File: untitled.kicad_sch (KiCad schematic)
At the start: 6 parts, among them J13 HDMI_A_1.4, J3 Bus_M.2_Socket_M, J5 USB3_A, J6 USB3_A, M1 M.2 Screw

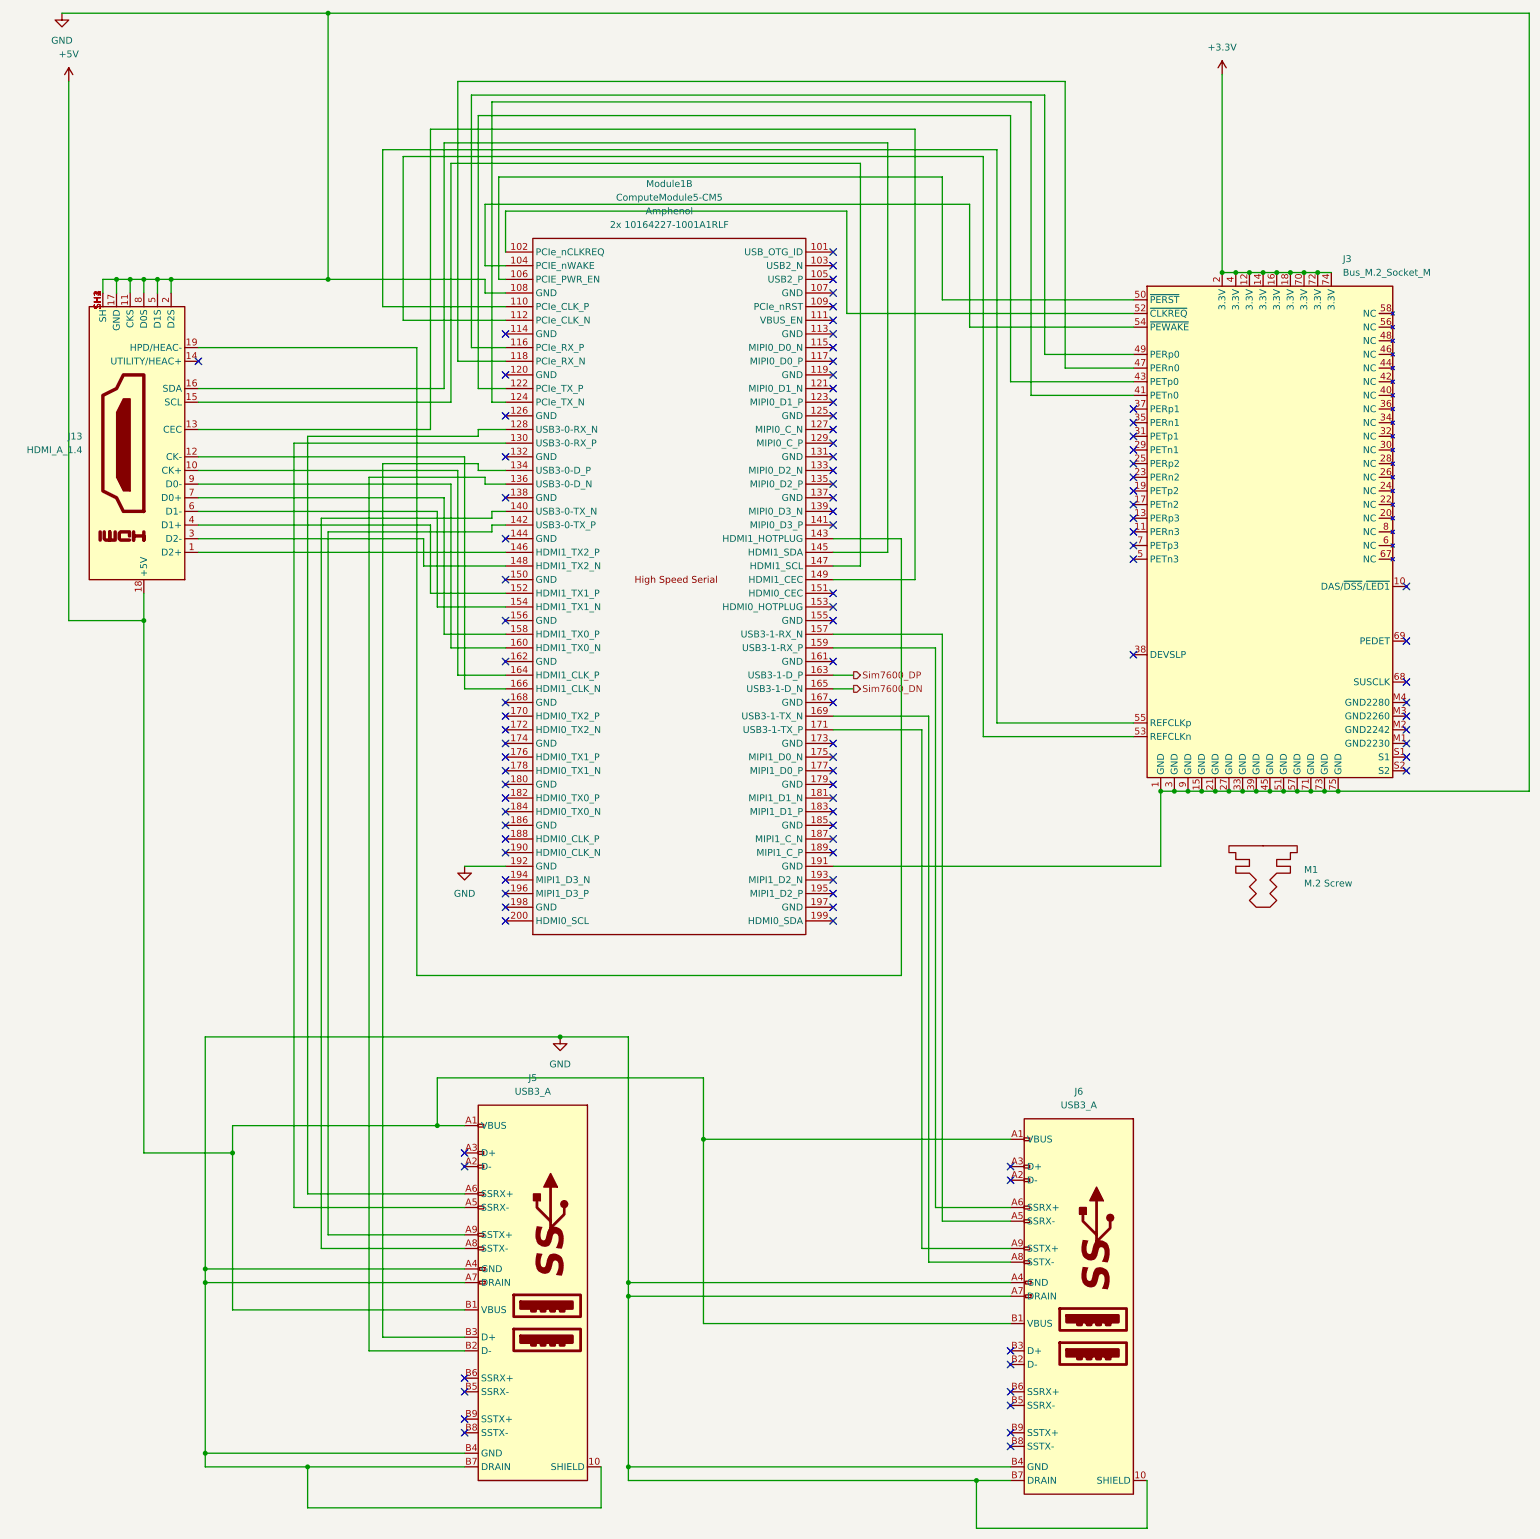
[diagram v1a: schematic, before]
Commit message: Work Changes and documentation
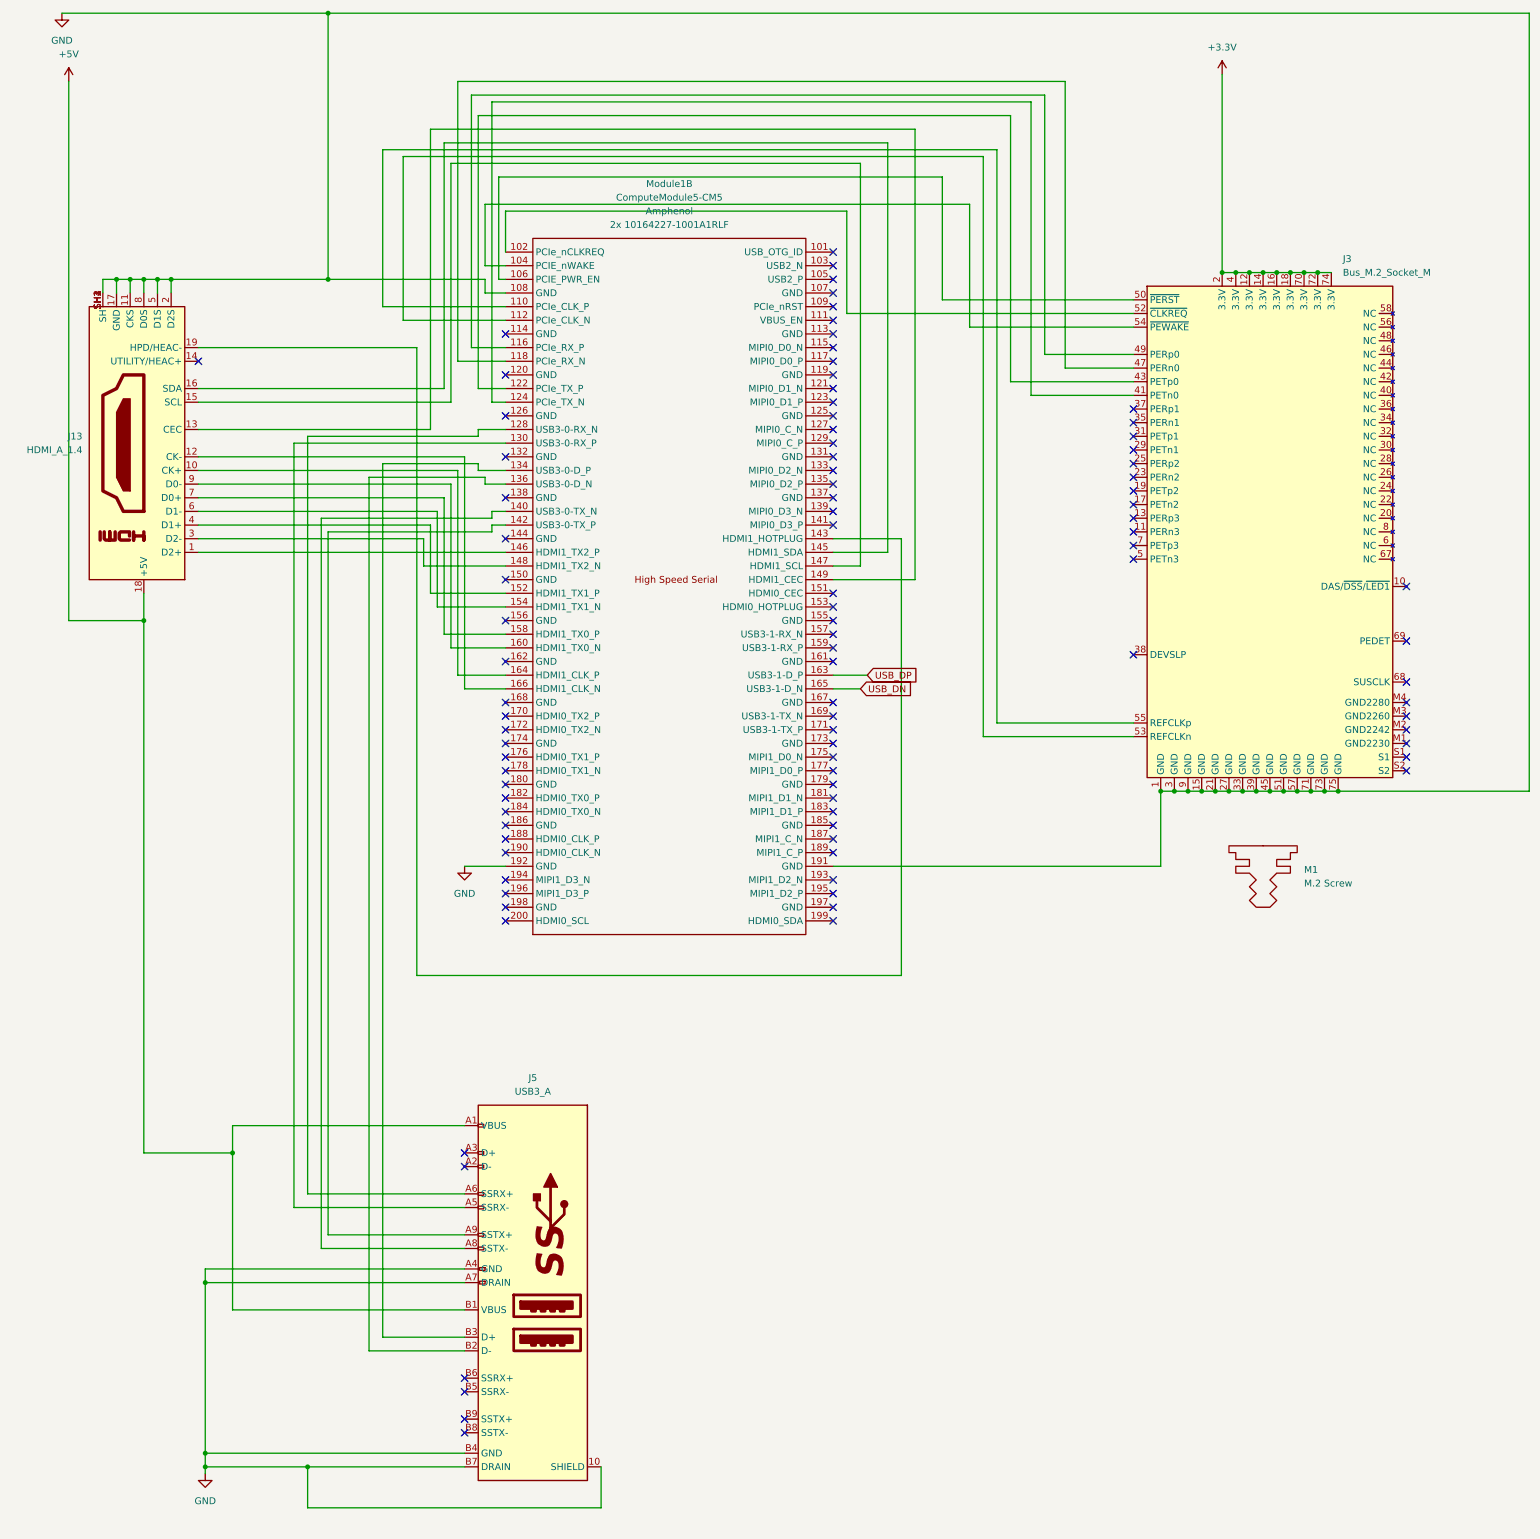
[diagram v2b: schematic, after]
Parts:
- removed J6: USB3_A, StackedUSBPretty:MOLEX_484060003, symbol Pi5Compute:USB3_A
- J5: footprint StackedUSBPretty:MOLEX_484060003 -> CM5IO:MTCONN_UBAF30-D2011
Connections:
- net Sim7600_DN renamed USB_DN
- net Sim7600_DP renamed USB_DP
- no-connect marks 101 -> 97
